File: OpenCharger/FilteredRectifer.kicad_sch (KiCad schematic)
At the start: 6 parts, among them Q1 IPT015N10N5, Q2 IPT015N10N5, Q3 IPT015N10N5, Q4 IPT015N10N5

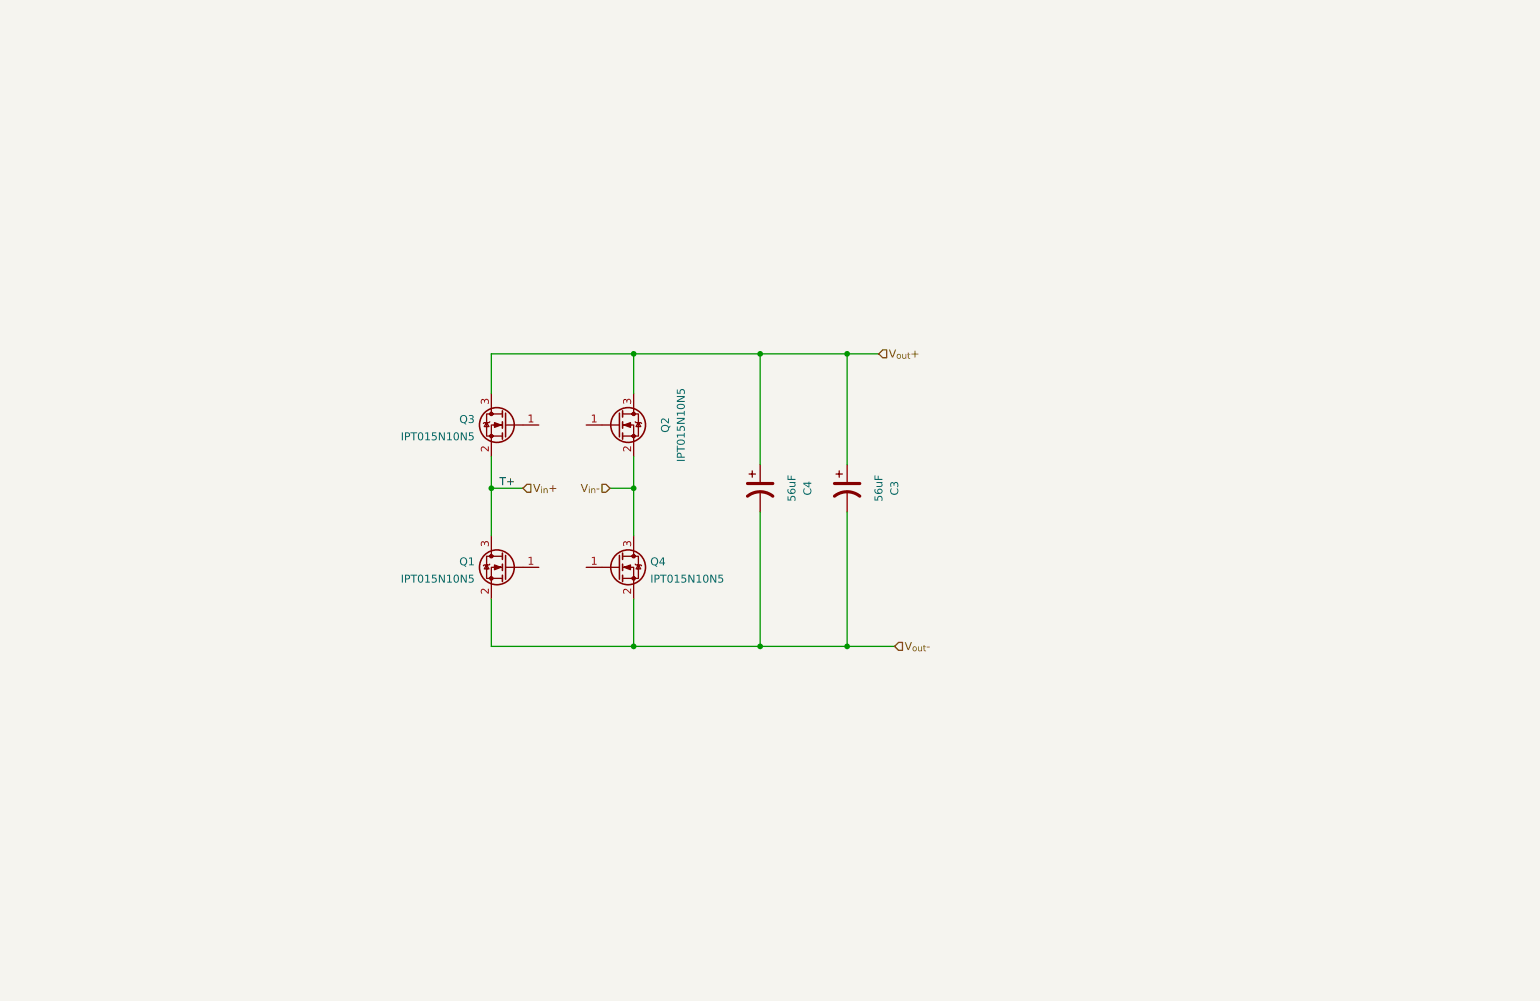
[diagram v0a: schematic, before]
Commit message: updated
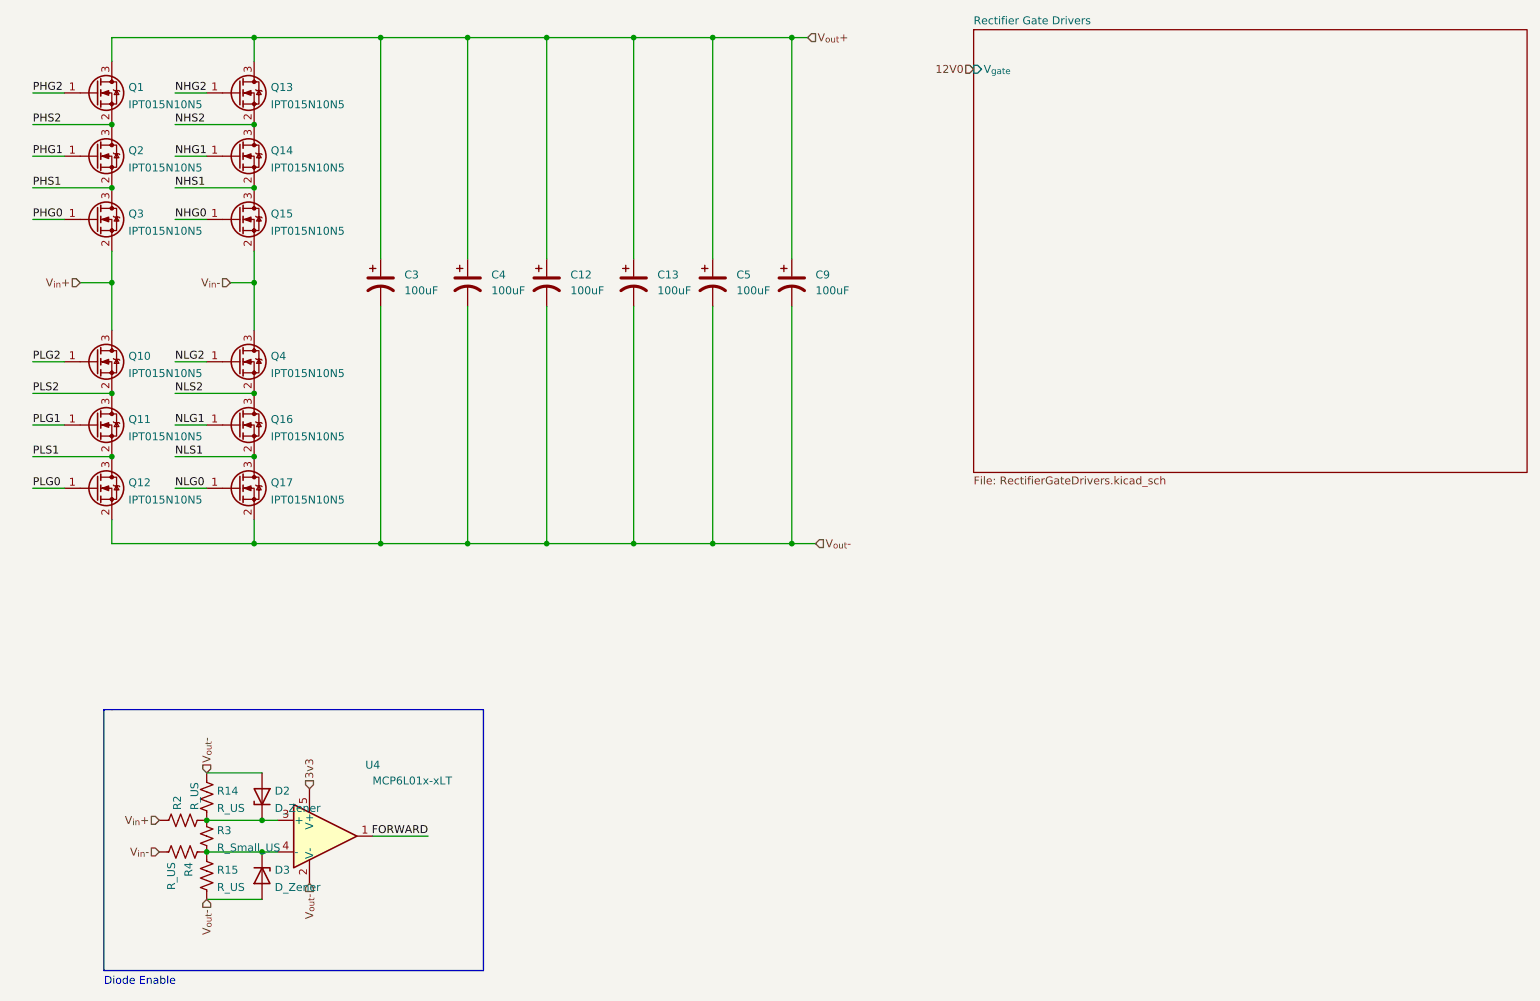
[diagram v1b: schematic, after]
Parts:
- added C12, C13, C5, C9: 100uF, Capacitor_THT:CP_Radial_D16.0mm_P7.50mm, symbol Device:C_Polarized_US
- added D2, D3: D_Zener, symbol Device:D_Zener
- added Q10, Q11, Q12, Q13, Q14, Q15, Q16, Q17: IPT015N10N5, Package_TO_SOT_SMD:Infineon_PG-HSOF-8-1, symbol Transistor_FET:IPT015N10N5
- added R14, R15, R2, R4: R_US, Resistor_SMD:R_0603_1608Metric, symbol Device:R_US
- added R3: R_Small_US, symbol Device:R_Small_US
- added U4: MCP6L01x-xLT, Package_TO_SOT_SMD:SOT-353_SC-70-5, symbol Amplifier_Operational:MCP6L01x-xLT
- C3, C4: value 56uF -> 100uF; footprint Capacitor_THT:CP_Radial_D40.0mm_P10.00mm_SnapIn -> Capacitor_THT:CP_Radial_D16.0mm_P7.50mm
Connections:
- net V_{in}+: now also Q10.3 (D), R2.1; no longer Q1.3 (D)
- net V_{in}-: now also Q15.2 (S), R4.2; no longer Q2.2 (S)
- net V_{out}+: now also Q1.3 (D), C12.1, C13.1, C5.1, C9.1, Q13.3 (D); no longer Q2.3 (D), Q3.3 (D)
- net V_{out}-: now also C12.2, C13.2, C5.2, C9.2, D2.2 (A), D3.2 (A), Q12.2 (S), Q17.2 (S), R14.2, R15.1, U4.2 (V-); no longer Q1.2 (S), Q4.2 (S)
- net PHG2: now reaches Q1.1 (G)
- net PHG0: now reaches Q3.1 (G)
- net NLG2: now reaches Q4.1 (G)
- net PHG1: now reaches Q2.1 (G)
- new net: D3.1 (K), R15.2, R3.2, R4.1, U4.4 (-)
- new net: D2.1 (K), R14.1, R2.2, R3.1, U4.3 (+)
- new net 3v3: U4.5 (V+)
- new net FORWARD: U4.1
- new net NHG0: Q15.1 (G)
- new net NHG1: Q14.1 (G)
- new net NHG2: Q13.1 (G)
- new net NHS1: Q14.2 (S), Q15.3 (D)
- new net NHS2: Q13.2 (S), Q14.3 (D)
- new net NLG0: Q17.1 (G)
- new net NLG1: Q16.1 (G)
- new net NLS1: Q16.2 (S), Q17.3 (D)
- new net NLS2: Q16.3 (D), Q4.2 (S)
- new net PHS1: Q2.2 (S), Q3.3 (D)
- new net PHS2: Q1.2 (S), Q2.3 (D)
- new net PLG0: Q12.1 (G)
- new net PLG1: Q11.1 (G)
- new net PLG2: Q10.1 (G)
- new net PLS1: Q11.2 (S), Q12.3 (D)
- new net PLS2: Q10.2 (S), Q11.3 (D)
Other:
- added sheet Rectifier Gate Drivers (RectifierGateDrivers.kicad_sch)
- note added: "Diode Enable"
- moved on the sheet: Q3, Q4
